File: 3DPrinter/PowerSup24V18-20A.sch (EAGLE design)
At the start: 2 parts, among them X1 CON-7.62-02P

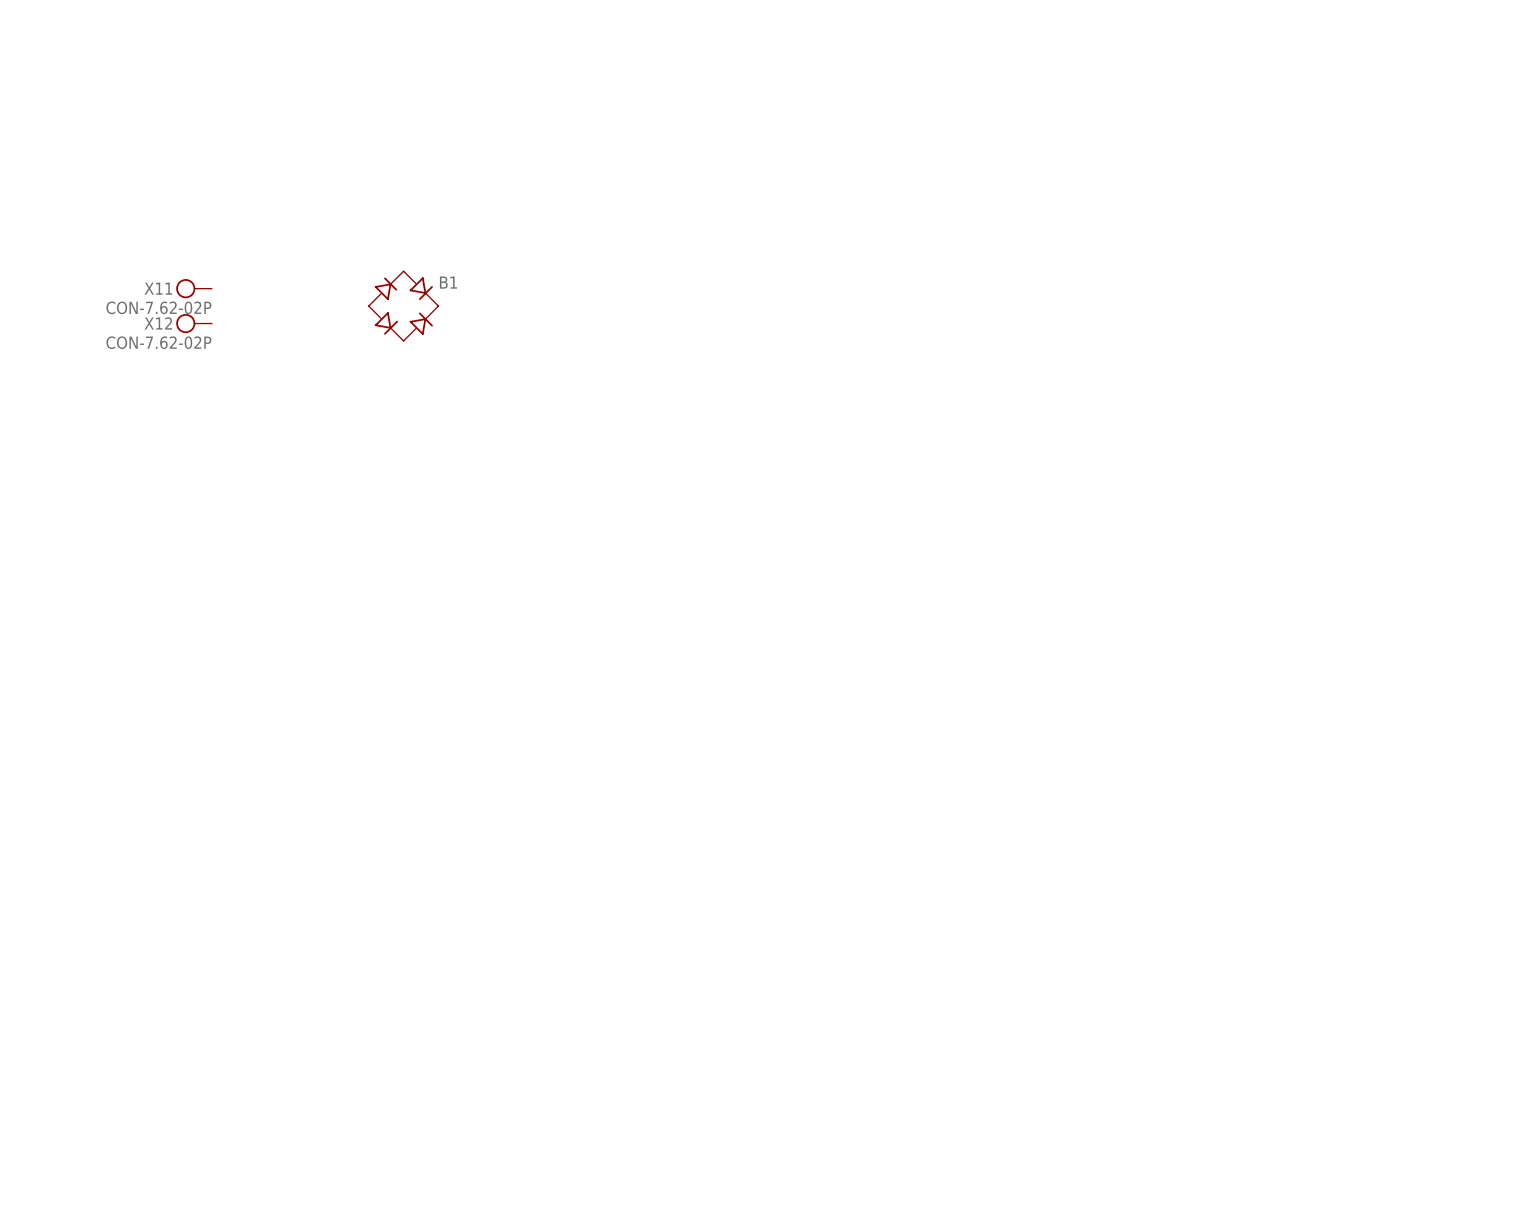
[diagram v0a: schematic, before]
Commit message: StandBy Supply
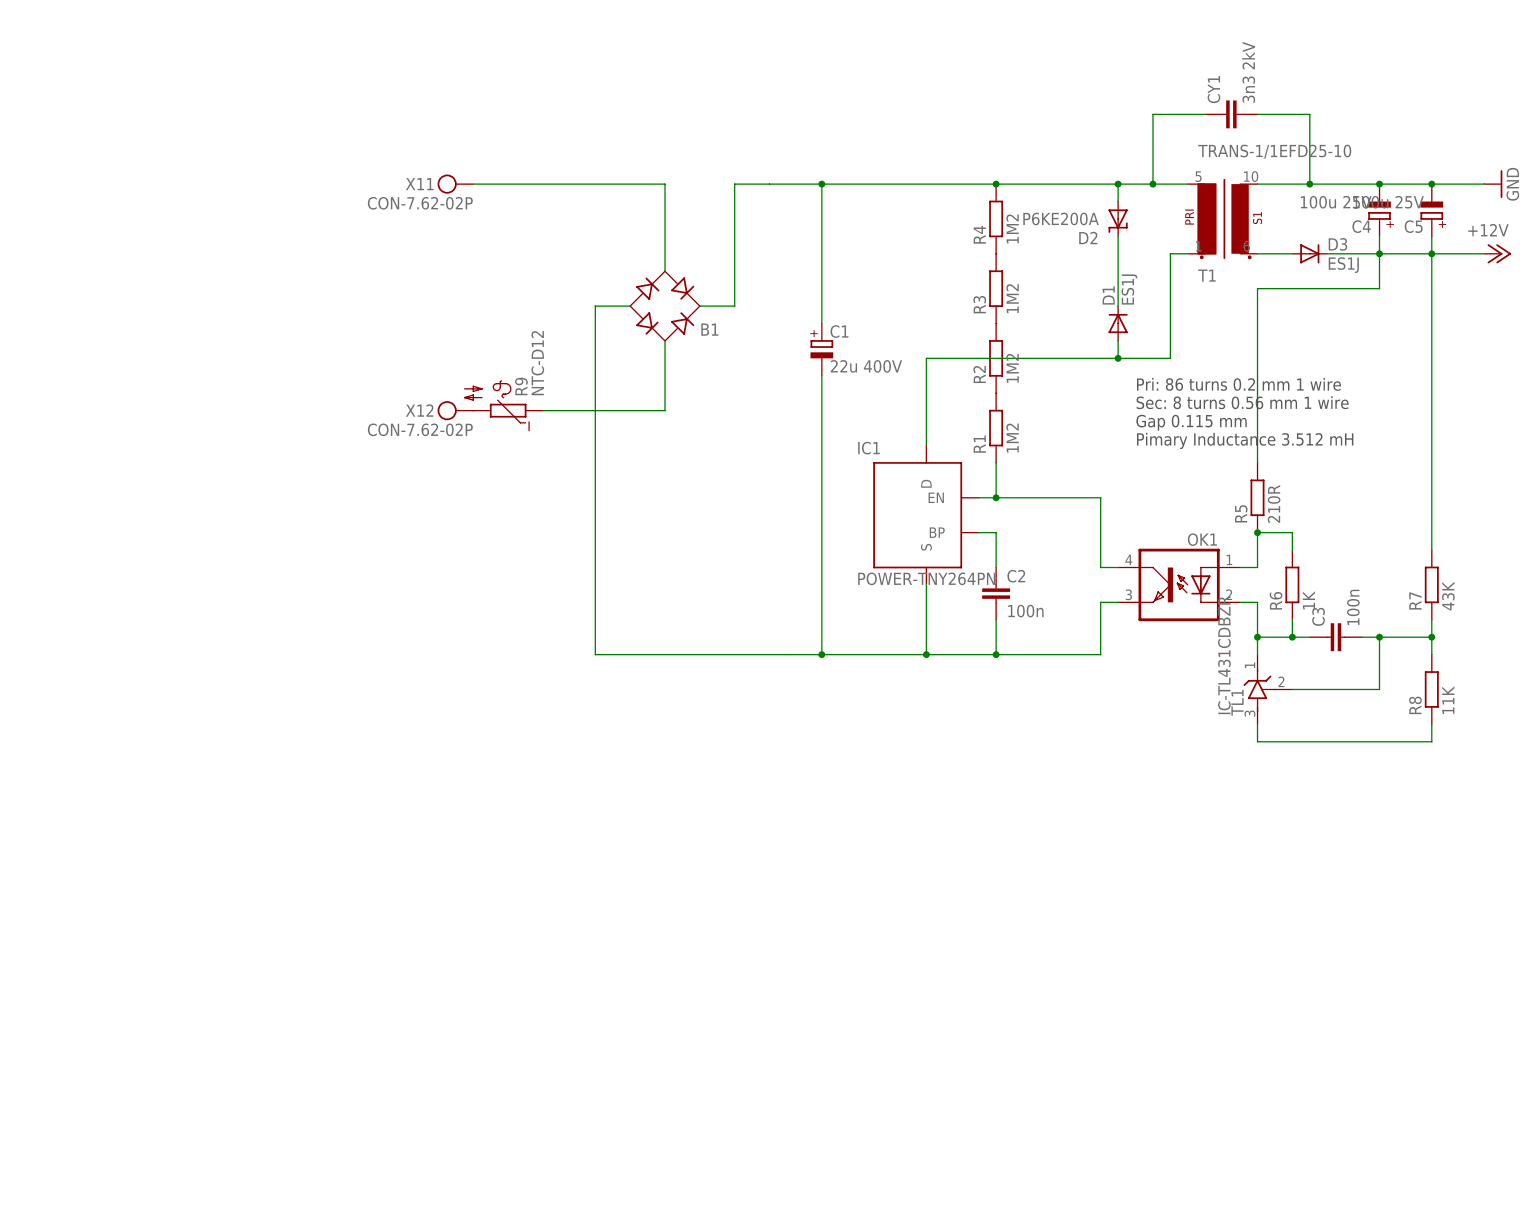
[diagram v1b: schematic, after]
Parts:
- added C1: 22u 400V, rcl:CPOL-EUE5-13
- added C2, C3: 100n, Namenlos:CAP_0805
- added C4, C5: 100u 25V, Namenlos:CAP-POL_E2.5-7
- added CY1: 3n3 2kV, rcl:CYYC7B5
- added D1, D3: ES1J, Namenlos:DIODE_ES1J
- added D2: P6KE200A, Namenlos:SUPRESSORDO-204AC
- added IC1: POWER-TNY264PN, Namenlos:POWER-TNY264PN
- added OK1: (no value), Namenlos:OPTOTRANSPC817
- added R1, R2, R3, R4: 1M2, Namenlos:R_0805
- added R5: 210R, Namenlos:R_0805
- added R6: 1K, Namenlos:R_0805
- added R7: 43K, Namenlos:R_0805
- added R8: 11K, Namenlos:R_0805
- added R9: NTC-D12, Namenlos:NTC-D12
- added T1: TRANS-1/1EFD25-10, Namenlos:TRANS-1/1EFD25-10
- added TL1: IC-TL431CDBZR, Namenlos:IC-TL431CDBZR
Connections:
- new net +12V: C4.+, C5.+, D3.C, R5.2, R7.2
- new net GND: C4.-, C5.-, CY1.2, T1.S1-2
- new net N$1: B1.AC2, X11.KL
- new net N$10: D1.C, D2.C
- new net N$11: C2.1, IC1.BP
- new net N$12: R9.2, X12.KL
- new net N$14: C3.1, OK1.C, R6.1, TL1.C
- new net N$15: OK1.A, R5.1, R6.2
- new net N$16: C3.2, R7.1, R8.2, TL1.R
- new net N$17: R8.1, TL1.A
- new net N$18: D3.A, T1.S1-1
- new net N$2: B1.AC1, R9.1
- new net N$3: B1.+, C1.+, CY1.1, D2.A, R4.2, T1.P1-2
- new net N$4: B1.-, C1.-, C2.2, IC1.S, OK1.EMIT
- new net N$5: R1.2, R2.1
- new net N$6: R2.2, R3.1
- new net N$7: R3.2, R4.1
- new net N$8: IC1.EN, OK1.COL, R1.1
- new net N$9: D1.A, IC1.D, T1.P1-1
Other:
- note added: "Pri: 86 turns 0.2 mm 1 wire Sec: 8 turns 0.56 mm 1 wire Gap 0.115 mm Pimary Inductance 3.512 mH"
- moved on the sheet: B1, X11, X12

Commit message: Something
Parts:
- added B2: (no value), Namenlos:RECTIFIERKBL
- added C10, C11, C6, C7, C8, C9: 100u 400V, rcl:CPOL-EUE7.5-18
- added C12, C13: 1u5 250V, rcl:C-EU225-074X268
- added C14: 1u 250V, rcl:C-EU225-074X268
- added R10: NTC-D12, Namenlos:NTC-D12
- added R11, R12: 160K, Namenlos:R_MF-0125
- added T2: _TRANSFORMERS_GDT_20X6.5, Namenlos:_TRANSFORMERS_GDT_20X6.5
- added U1: SG3525AN, Namenlos:SG3525AN
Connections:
- new net AC1: B1.AC2, B2.AC2, X11.KL
- new net AC2: R10.2, R9.2, X12.KL
- new net N$13: B2.+, C10.+, C11.+, C12.1, C6.+, C7.+, C8.+, C9.+, R12.2
- new net N$19: B2.-, C10.-, C11.-, C13.2, C6.-, C7.-, C8.-, C9.-, R11.1
- new net N$20: T2.P1-1, U1.OUT_A
- new net N$21: T2.P1-2, U1.OUT_B
- net N$1: now also B2.AC1, R10.1; no longer B1.AC2, X11.KL
- net N$12: now also C12.2, C13.1, C14.1, R11.2, R12.1; no longer R9.2, X12.KL

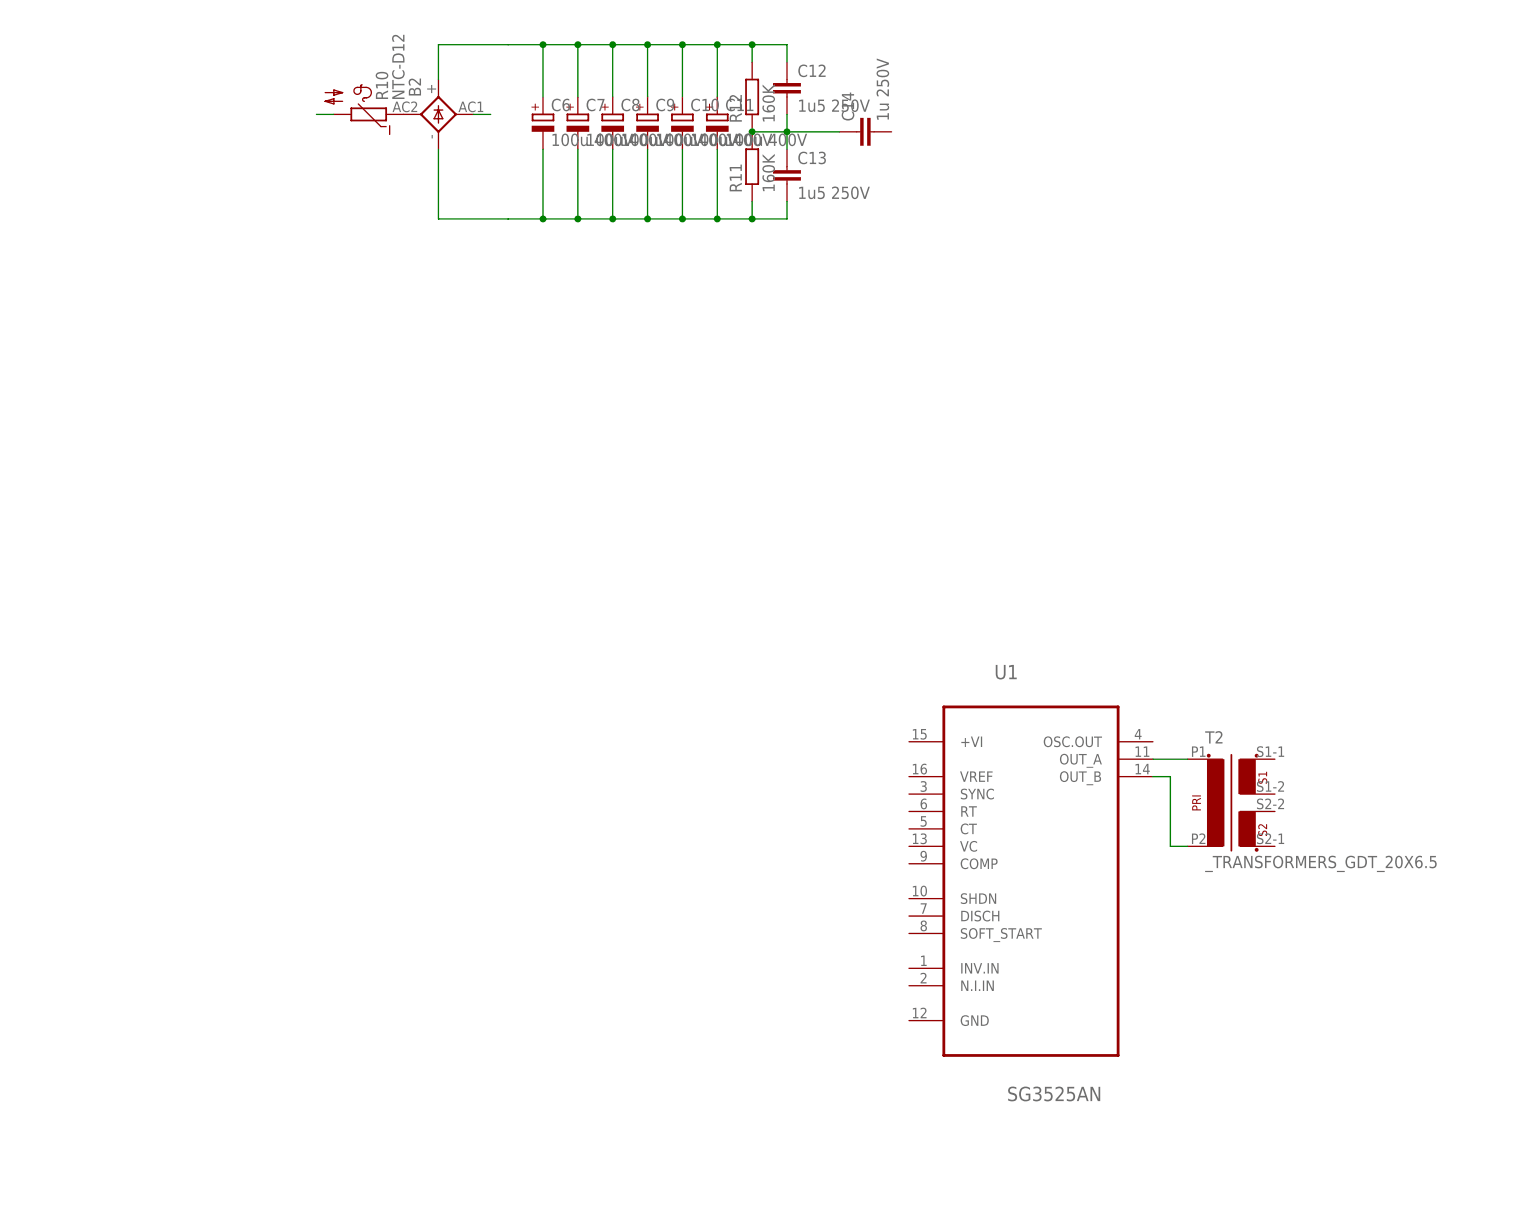
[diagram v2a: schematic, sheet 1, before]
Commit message: Горячая сторона
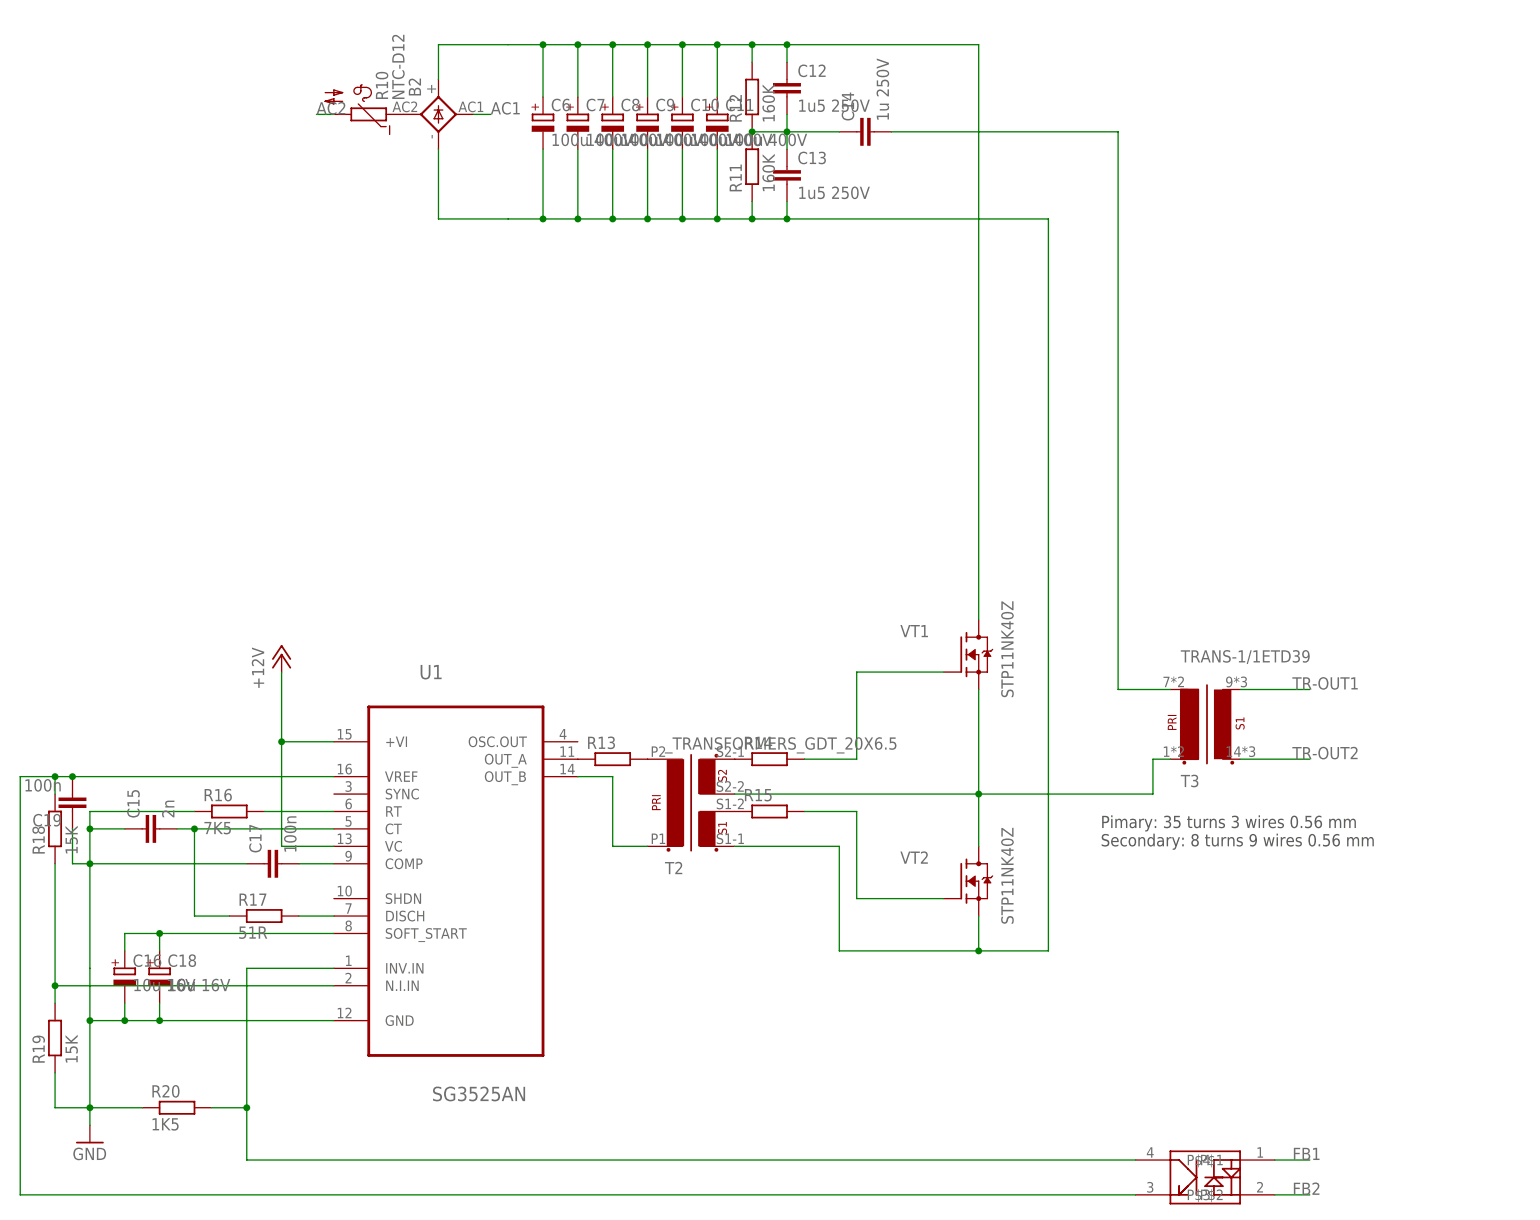
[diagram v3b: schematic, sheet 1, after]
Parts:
- added C15: 2n, Namenlos:CAP_0805
- added C16, C18: 10u 16V, Namenlos:CAP-POL_3528
- added C17, C19: 100n, Namenlos:CAP_0805
- added R13, R14, R15: (no value), Namenlos:R_1206
- added R16: 7K5, Namenlos:R_0805
- added R17: 51R, Namenlos:R_0805
- added R18, R19: 15K, Namenlos:R_0805
- added R20: 1K5, Namenlos:R_0805
- added T3: TRANS-1/1ETD39, Namenlos:TRANS-1/1ETD39
- added U$1: OPTO-EL3H4(TA)-VG, Namenlos:OPTO-EL3H4(TA)-VG
- added VT1, VT2: STP11NK40Z, Namenlos:FET-NTO-220
- C1: value 22u 400V -> 100u 400V; device rcl:CPOL-EUE5-13 -> rcl:CPOL-EUE7.5-18
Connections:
- new net FB1: U$1.P$1
- new net FB2: U$1.P$2
- new net N$22: R13.2, T2.P1-2
- new net N$23: R14.1, T2.S2-1
- new net N$24: R15.1, T2.S1-2
- new net N$25: R14.2, VT1.G
- new net N$26: R15.2, VT2.G
- new net N$27: T2.S2-2, T3.P1-1, VT1.S, VT2.D
- new net N$28: C14.2, T3.P1-2
- new net N$29: R16.2, U1.RT
- new net N$30: C15.2, R17.1, U1.CT
- new net N$31: C19.2, R18.2, U$1.P$3, U1.VREF
- new net N$32: R17.2, U1.DISCH
- new net N$33: C16.+, C18.+, U1.SOFT_START
- new net N$34: R18.1, R19.2, U1.N.I.IN
- new net N$35: C17.2, U1.COMP
- new net N$36: R20.2, U$1.P$4, U1.INV.IN
- new net TR-OUT1: T3.S1-2
- new net TR-OUT2: T3.S1-1
- net +12V: now also U1.+VI, U1.VC
- net GND: now also C15.1, C16.-, C17.1, C18.-, C19.1, R16.1, R19.1, R20.1, U1.GND
- net N$13: now also VT1.D
- net N$19: now also T2.S1-1, VT2.S
- net N$20: now also R13.1; no longer T2.P1-1
- net N$21: now also T2.P1-1; no longer T2.P1-2
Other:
- note added: "Pimary: 35 turns 3 wires 0.56 mm Secondary: 8 turns 9 wires 0.56 mm"
- moved on the sheet: T2, U1
